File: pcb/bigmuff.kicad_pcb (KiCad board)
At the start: 2 copper layers, 46 parts, among them Q1 BC549, Q2 BC549, Q3 BC549, Q4 BC549

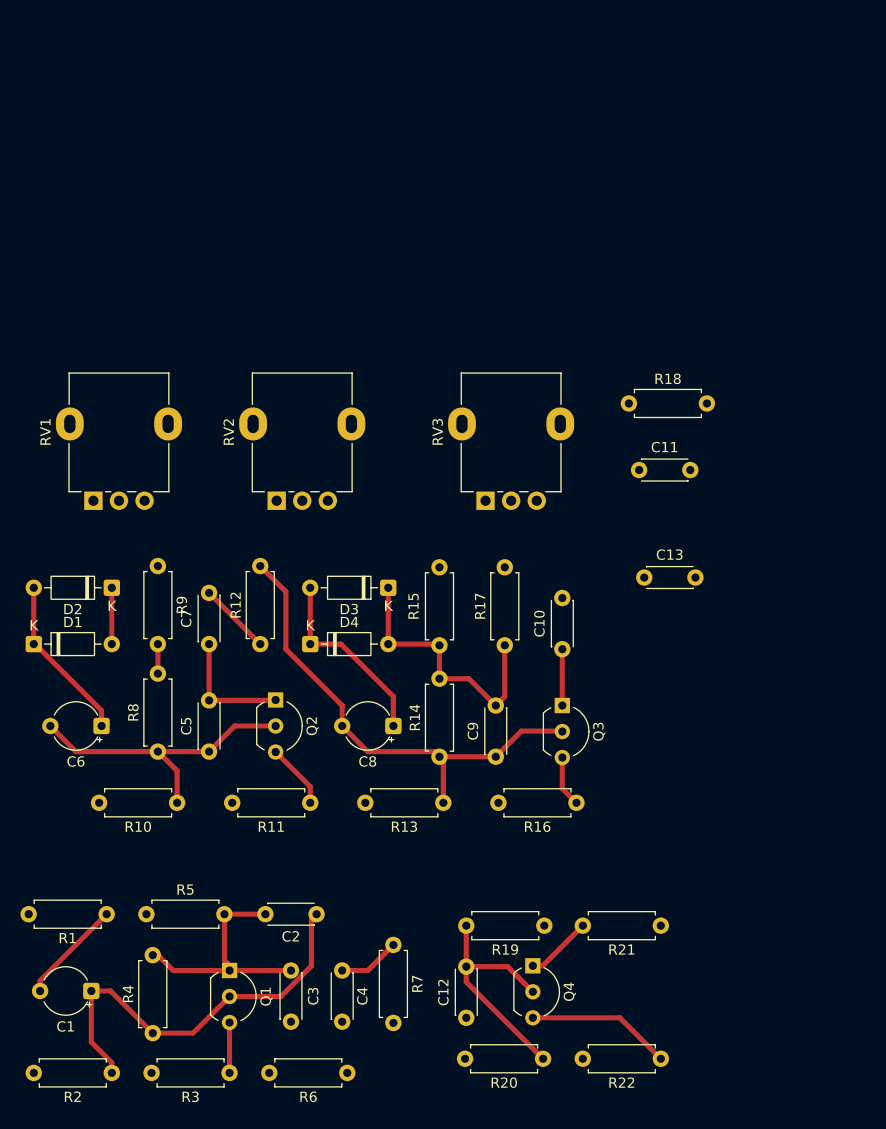
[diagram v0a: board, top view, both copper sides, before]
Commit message: pcb update
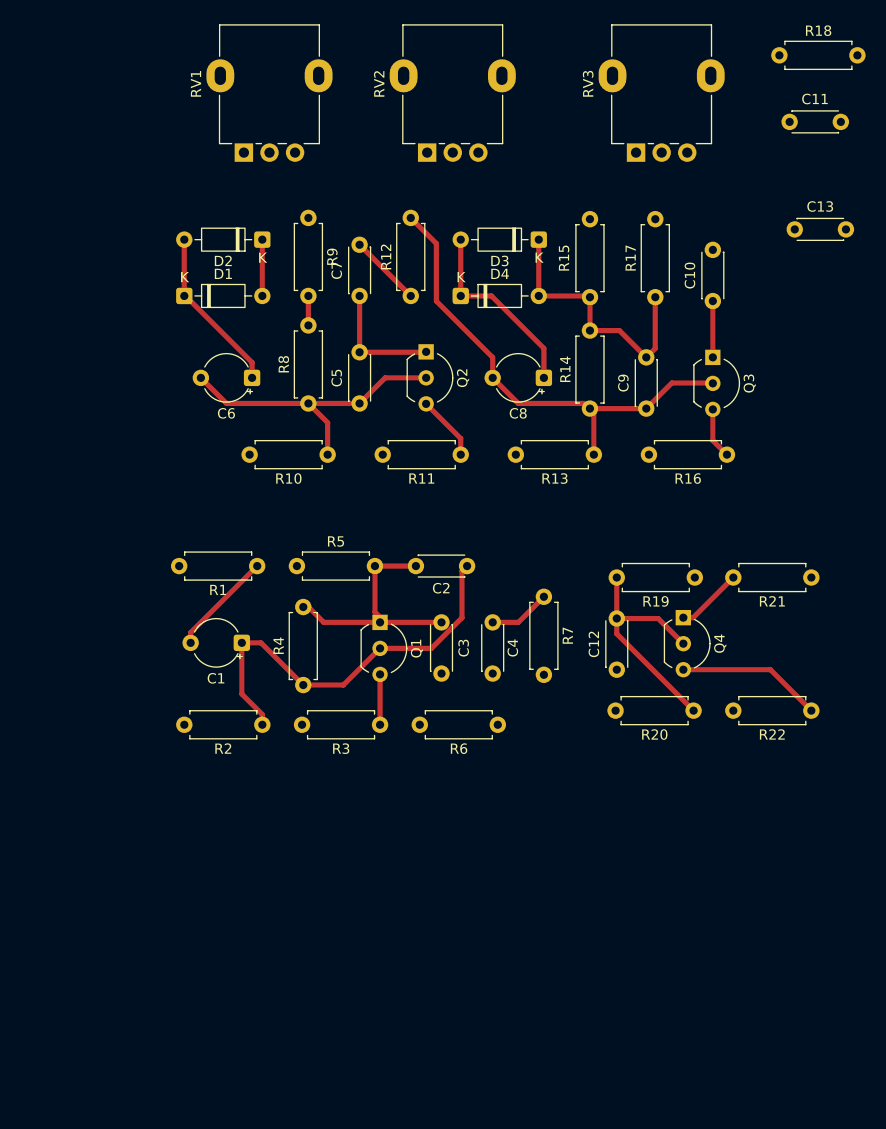
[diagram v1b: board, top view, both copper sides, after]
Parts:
- moved Q2 37.0 mm to (110.2, 95.0)
- moved R16 37.0 mm to (139.6, 105.0)
- moved R17 37.0 mm to (132.6, 89.6)
- moved C1 37.0 mm to (92.2, 123.4)
- moved C10 37.0 mm to (138.2, 90.0)
- moved C11 37.0 mm to (145.7, 72.5)
- moved C12 37.0 mm to (128.8, 126.0)
- moved C13 37.0 mm to (146.2, 83.0)
- moved C2 37.0 mm to (114.2, 115.9)
- moved C3 37.0 mm to (111.7, 121.4)
- moved C4 37.0 mm to (116.7, 126.4)
- moved C5 37.0 mm to (103.7, 100.0)
- moved C6 37.0 mm to (93.2, 97.5)
- moved C7 37.0 mm to (103.7, 89.5)
- moved C8 37.0 mm to (121.7, 97.5)
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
